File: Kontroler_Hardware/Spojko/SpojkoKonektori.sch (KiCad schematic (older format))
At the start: 14 parts, among them J3 CONN_02X40, J4 CONN_02X40, J5 CONN_02X40, J6 CONN_02X40, J7 CONN_02X40, J8 CONN_02X40

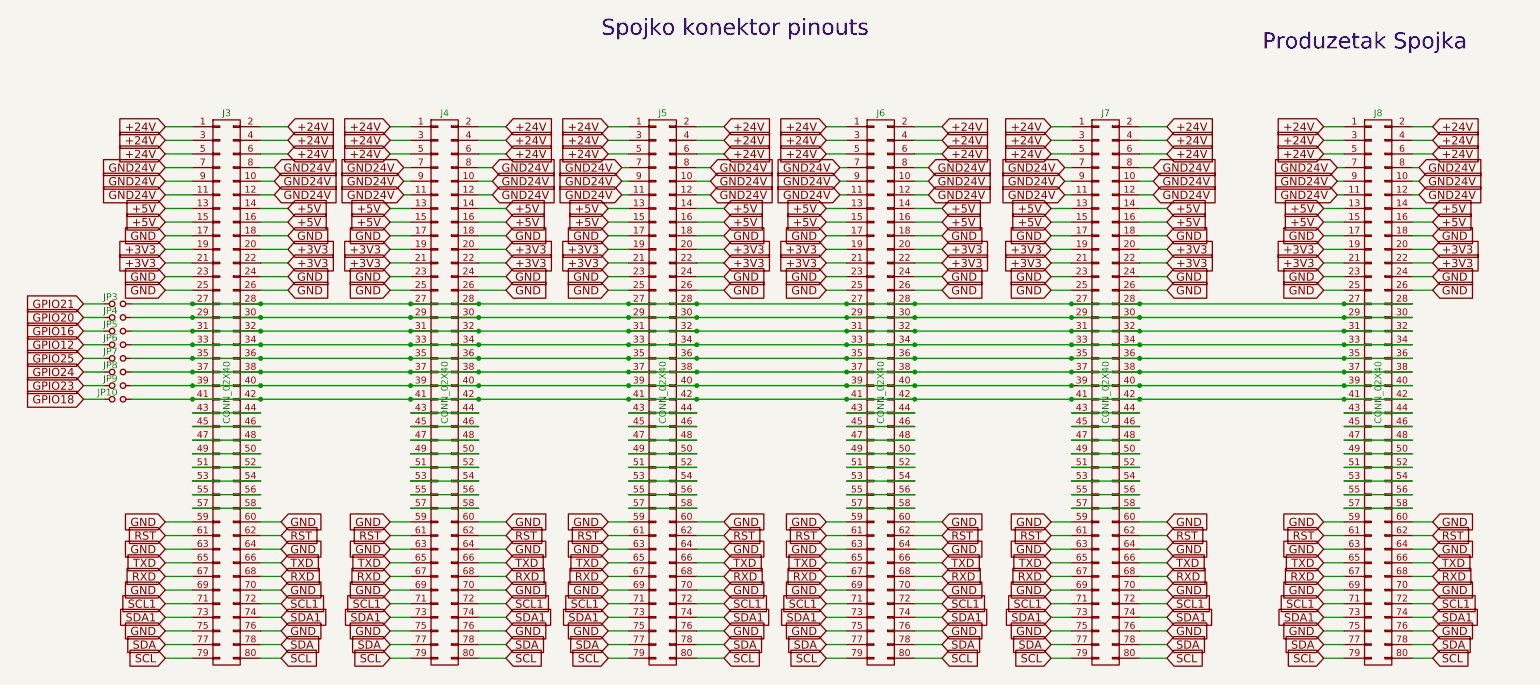
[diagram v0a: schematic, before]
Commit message: NewTemplates
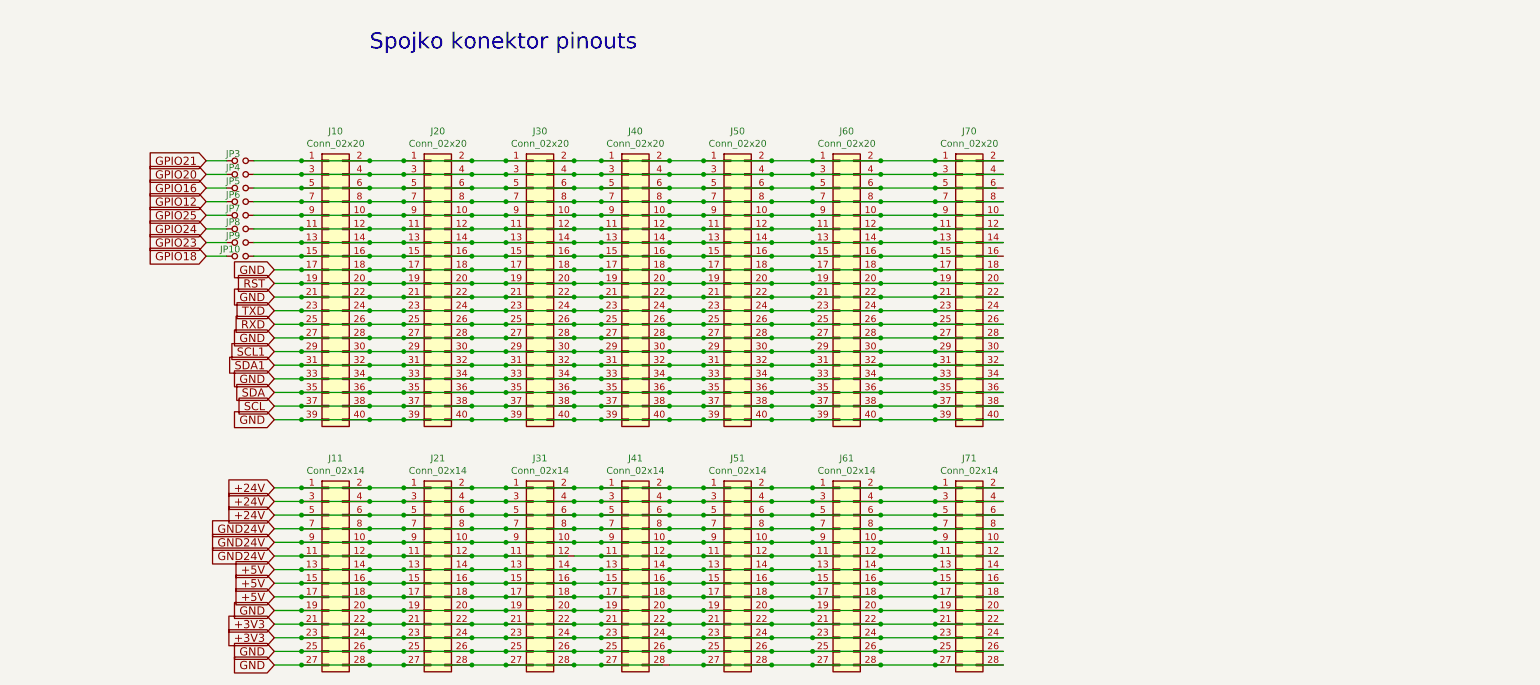
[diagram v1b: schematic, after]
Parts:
- removed J3, J4, J5, J6, J7: CONN_02X40, Pin_Headers:Pin_Header_Straight_2x40_Pitch2.54mm, symbol Spojko-rescue:CONN_02X40
- removed J8: CONN_02X40, Pin_Headers:Pin_Header_Angled_2x40_Pitch2.54mm, symbol Spojko-rescue:CONN_02X40
- added J10, J20, J30, J40, J50, J60: Conn_02x20, Connector_PinHeader_2.54mm:PinHeader_2x20_P2.54mm_Vertical, symbol Spojko-rescue:Conn_02x20_Odd_Even-Connector_Generic
- added J11, J21, J31, J41, J51, J61: Conn_02x14, Connector_PinHeader_2.54mm:PinHeader_2x14_P2.54mm_Vertical, symbol Spojko-rescue:Conn_02x14_Odd_Even-Connector_Generic
- added J70: Conn_02x20, Connector_PinHeader_2.54mm:PinHeader_2x20_P2.54mm_Horizontal, symbol Spojko-rescue:Conn_02x20_Odd_Even-Connector_Generic
- added J71: Conn_02x14, Connector_PinHeader_2.54mm:PinHeader_2x14_P2.54mm_Horizontal, symbol Spojko-rescue:Conn_02x14_Odd_Even-Connector_Generic
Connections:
- net +24V: now also J11.1 (Pin_1), J11.2 (Pin_2), J11.3 (Pin_3), J11.4 (Pin_4), J11.5 (Pin_5), J11.6 (Pin_6), J21.1 (Pin_1), J21.2 (Pin_2), J21.3 (Pin_3), J21.4 (Pin_4), J21.5 (Pin_5), J21.6 (Pin_6), J31.1 (Pin_1), J31.2 (Pin_2), J31.3 (Pin_3), J31.4 (Pin_4), J31.5 (Pin_5), J31.6 (Pin_6), J41.1 (Pin_1), J41.2 (Pin_2), J41.3 (Pin_3), J41.4 (Pin_4), J41.5 (Pin_5), J41.6 (Pin_6), J51.1 (Pin_1), J51.2 (Pin_2), J51.3 (Pin_3), J51.4 (Pin_4), J51.5 (Pin_5), J51.6 (Pin_6), J61.1 (Pin_1), J61.2 (Pin_2), J61.3 (Pin_3), J61.4 (Pin_4), J61.5 (Pin_5), J61.6 (Pin_6), J71.1 (Pin_1), J71.2 (Pin_2), J71.3 (Pin_3), J71.4 (Pin_4), J71.5 (Pin_5), J71.6 (Pin_6)
- net +3V3: now also J11.21 (Pin_21), J11.22 (Pin_22), J11.23 (Pin_23), J11.24 (Pin_24), J21.21 (Pin_21), J21.22 (Pin_22), J21.23 (Pin_23), J21.24 (Pin_24), J31.21 (Pin_21), J31.22 (Pin_22), J31.23 (Pin_23), J31.24 (Pin_24), J41.21 (Pin_21), J41.22 (Pin_22), J41.23 (Pin_23), J41.24 (Pin_24), J51.21 (Pin_21), J51.22 (Pin_22), J51.23 (Pin_23), J51.24 (Pin_24), J61.21 (Pin_21), J61.22 (Pin_22), J61.23 (Pin_23), J61.24 (Pin_24), J71.21 (Pin_21), J71.22 (Pin_22), J71.23 (Pin_23), J71.24 (Pin_24)
- net +5V: now also J11.13 (Pin_13), J11.14 (Pin_14), J11.15 (Pin_15), J11.16 (Pin_16), J11.17 (Pin_17), J11.18 (Pin_18), J21.13 (Pin_13), J21.14 (Pin_14), J21.15 (Pin_15), J21.16 (Pin_16), J21.17 (Pin_17), J21.18 (Pin_18), J31.13 (Pin_13), J31.14 (Pin_14), J31.15 (Pin_15), J31.16 (Pin_16), J31.17 (Pin_17), J31.18 (Pin_18), J41.13 (Pin_13), J41.14 (Pin_14), J41.15 (Pin_15), J41.16 (Pin_16), J41.17 (Pin_17), J41.18 (Pin_18), J51.13 (Pin_13), J51.14 (Pin_14), J51.15 (Pin_15), J51.16 (Pin_16), J51.17 (Pin_17), J51.18 (Pin_18), J61.13 (Pin_13), J61.14 (Pin_14), J61.15 (Pin_15), J61.16 (Pin_16), J61.17 (Pin_17), J61.18 (Pin_18), J71.13 (Pin_13), J71.14 (Pin_14), J71.15 (Pin_15), J71.16 (Pin_16), J71.17 (Pin_17), J71.18 (Pin_18)
- net GND: now also J10.17 (Pin_17), J10.18 (Pin_18), J10.21 (Pin_21), J10.22 (Pin_22), J10.27 (Pin_27), J10.28 (Pin_28), J10.33 (Pin_33), J10.34 (Pin_34), J10.39 (Pin_39), J10.40 (Pin_40), J11.19 (Pin_19), J11.20 (Pin_20), J11.25 (Pin_25), J11.26 (Pin_26), J11.27 (Pin_27), J11.28 (Pin_28), J20.17 (Pin_17), J20.18 (Pin_18), J20.21 (Pin_21), J20.22 (Pin_22), J20.27 (Pin_27), J20.28 (Pin_28), J20.33 (Pin_33), J20.34 (Pin_34), J20.39 (Pin_39), J20.40 (Pin_40), J21.19 (Pin_19), J21.20 (Pin_20), J21.25 (Pin_25), J21.26 (Pin_26), J21.27 (Pin_27), J21.28 (Pin_28), J30.17 (Pin_17), J30.18 (Pin_18), J30.21 (Pin_21), J30.22 (Pin_22), J30.27 (Pin_27), J30.28 (Pin_28), J30.33 (Pin_33), J30.34 (Pin_34), J30.39 (Pin_39), J30.40 (Pin_40), J31.19 (Pin_19), J31.20 (Pin_20), J31.25 (Pin_25), J31.26 (Pin_26), J31.27 (Pin_27), J31.28 (Pin_28), J40.17 (Pin_17), J40.18 (Pin_18), J40.21 (Pin_21), J40.22 (Pin_22), J40.27 (Pin_27), J40.28 (Pin_28), J40.33 (Pin_33), J40.34 (Pin_34), J40.39 (Pin_39), J40.40 (Pin_40), J41.19 (Pin_19), J41.20 (Pin_20), J41.25 (Pin_25), J41.26 (Pin_26), J41.27 (Pin_27), J50.17 (Pin_17), J50.18 (Pin_18), J50.21 (Pin_21), J50.22 (Pin_22), J50.27 (Pin_27), J50.28 (Pin_28), J50.33 (Pin_33), J50.34 (Pin_34), J50.39 (Pin_39), J50.40 (Pin_40), J51.19 (Pin_19), J51.20 (Pin_20), J51.25 (Pin_25), J51.26 (Pin_26), J60.17 (Pin_17), J60.18 (Pin_18), J60.21 (Pin_21), J60.22 (Pin_22), J60.27 (Pin_27), J60.28 (Pin_28), J60.33 (Pin_33), J60.34 (Pin_34), J60.39 (Pin_39), J60.40 (Pin_40), J61.19 (Pin_19), J61.20 (Pin_20), J61.25 (Pin_25), J61.26 (Pin_26), J70.17 (Pin_17), J70.18 (Pin_18), J70.21 (Pin_21), J70.22 (Pin_22), J70.27 (Pin_27), J70.28 (Pin_28), J70.33 (Pin_33), J70.34 (Pin_34), J70.39 (Pin_39), J70.40 (Pin_40), J71.19 (Pin_19), J71.20 (Pin_20), J71.25 (Pin_25), J71.26 (Pin_26)
- net GND24V: now also J11.10 (Pin_10), J11.11 (Pin_11), J11.12 (Pin_12), J11.7 (Pin_7), J11.8 (Pin_8), J11.9 (Pin_9), J21.10 (Pin_10), J21.11 (Pin_11), J21.12 (Pin_12), J21.7 (Pin_7), J21.8 (Pin_8), J21.9 (Pin_9), J31.10 (Pin_10), J31.11 (Pin_11), J31.7 (Pin_7), J31.8 (Pin_8), J31.9 (Pin_9), J41.10 (Pin_10), J41.7 (Pin_7), J41.8 (Pin_8), J41.9 (Pin_9), J51.10 (Pin_10), J51.7 (Pin_7), J51.8 (Pin_8), J51.9 (Pin_9), J61.10 (Pin_10), J61.7 (Pin_7), J61.8 (Pin_8), J61.9 (Pin_9), J71.10 (Pin_10), J71.7 (Pin_7), J71.8 (Pin_8), J71.9 (Pin_9)
- net RST: now also J10.19 (Pin_19), J10.20 (Pin_20), J20.19 (Pin_19), J20.20 (Pin_20), J30.19 (Pin_19), J30.20 (Pin_20), J40.19 (Pin_19), J40.20 (Pin_20), J50.19 (Pin_19), J50.20 (Pin_20), J60.19 (Pin_19), J60.20 (Pin_20), J70.19 (Pin_19), J70.20 (Pin_20)
- net RXD: now also J10.25 (Pin_25), J10.26 (Pin_26), J20.25 (Pin_25), J20.26 (Pin_26), J30.25 (Pin_25), J30.26 (Pin_26), J40.25 (Pin_25), J40.26 (Pin_26), J50.25 (Pin_25), J50.26 (Pin_26), J60.25 (Pin_25), J60.26 (Pin_26), J70.25 (Pin_25), J70.26 (Pin_26)
- net SCL: now also J10.37 (Pin_37), J10.38 (Pin_38), J20.37 (Pin_37), J20.38 (Pin_38), J30.37 (Pin_37), J30.38 (Pin_38), J40.37 (Pin_37), J40.38 (Pin_38), J50.37 (Pin_37), J50.38 (Pin_38), J60.37 (Pin_37), J60.38 (Pin_38), J70.37 (Pin_37), J70.38 (Pin_38)
- net SCL1: now also J10.29 (Pin_29), J10.30 (Pin_30), J20.29 (Pin_29), J20.30 (Pin_30), J30.29 (Pin_29), J30.30 (Pin_30), J40.29 (Pin_29), J40.30 (Pin_30), J50.29 (Pin_29), J50.30 (Pin_30), J60.29 (Pin_29), J60.30 (Pin_30), J70.29 (Pin_29), J70.30 (Pin_30)
- net SDA: now also J10.35 (Pin_35), J10.36 (Pin_36), J20.35 (Pin_35), J20.36 (Pin_36), J30.35 (Pin_35), J30.36 (Pin_36), J40.35 (Pin_35), J40.36 (Pin_36), J50.35 (Pin_35), J50.36 (Pin_36), J60.35 (Pin_35), J60.36 (Pin_36), J70.35 (Pin_35), J70.36 (Pin_36)
- net SDA1: now also J10.31 (Pin_31), J10.32 (Pin_32), J20.31 (Pin_31), J20.32 (Pin_32), J30.31 (Pin_31), J30.32 (Pin_32), J40.31 (Pin_31), J40.32 (Pin_32), J50.31 (Pin_31), J50.32 (Pin_32), J60.31 (Pin_31), J60.32 (Pin_32), J70.31 (Pin_31), J70.32 (Pin_32)
- net TXD: now also J10.23 (Pin_23), J10.24 (Pin_24), J20.23 (Pin_23), J20.24 (Pin_24), J30.23 (Pin_23), J30.24 (Pin_24), J40.23 (Pin_23), J40.24 (Pin_24), J50.23 (Pin_23), J50.24 (Pin_24), J60.23 (Pin_23), J60.24 (Pin_24), J70.23 (Pin_23), J70.24 (Pin_24)
- net at JP3.2: now also J10.1 (Pin_1), J10.2 (Pin_2), J20.1 (Pin_1), J20.2 (Pin_2), J30.1 (Pin_1), J30.2 (Pin_2), J40.1 (Pin_1), J40.2 (Pin_2), J50.1 (Pin_1), J50.2 (Pin_2), J60.1 (Pin_1), J60.2 (Pin_2), J70.1 (Pin_1), J70.2 (Pin_2)
- net at JP4.2: now also J10.3 (Pin_3), J10.4 (Pin_4), J20.3 (Pin_3), J20.4 (Pin_4), J30.3 (Pin_3), J30.4 (Pin_4), J40.3 (Pin_3), J40.4 (Pin_4), J50.3 (Pin_3), J50.4 (Pin_4), J60.3 (Pin_3), J60.4 (Pin_4), J70.3 (Pin_3), J70.4 (Pin_4)
- net at JP5.2: now also J10.5 (Pin_5), J10.6 (Pin_6), J20.5 (Pin_5), J20.6 (Pin_6), J30.5 (Pin_5), J30.6 (Pin_6), J40.5 (Pin_5), J40.6 (Pin_6), J50.5 (Pin_5), J50.6 (Pin_6), J60.5 (Pin_5), J60.6 (Pin_6), J70.5 (Pin_5)
- net at JP6.2: now also J10.7 (Pin_7), J10.8 (Pin_8), J20.7 (Pin_7), J20.8 (Pin_8), J30.7 (Pin_7), J30.8 (Pin_8), J40.7 (Pin_7), J40.8 (Pin_8), J50.7 (Pin_7), J50.8 (Pin_8), J60.7 (Pin_7), J60.8 (Pin_8), J70.7 (Pin_7), J70.8 (Pin_8)
- net at JP7.2: now also J10.10 (Pin_10), J10.9 (Pin_9), J20.10 (Pin_10), J20.9 (Pin_9), J30.10 (Pin_10), J30.9 (Pin_9), J40.10 (Pin_10), J40.9 (Pin_9), J50.10 (Pin_10), J50.9 (Pin_9), J60.10 (Pin_10), J60.9 (Pin_9), J70.10 (Pin_10), J70.9 (Pin_9)
- net at JP8.2: now also J10.11 (Pin_11), J10.12 (Pin_12), J20.11 (Pin_11), J20.12 (Pin_12), J30.11 (Pin_11), J30.12 (Pin_12), J40.11 (Pin_11), J40.12 (Pin_12), J50.11 (Pin_11), J50.12 (Pin_12), J60.11 (Pin_11), J60.12 (Pin_12), J70.11 (Pin_11), J70.12 (Pin_12)
- net at JP9.2: now also J10.13 (Pin_13), J10.14 (Pin_14), J20.13 (Pin_13), J20.14 (Pin_14), J30.13 (Pin_13), J30.14 (Pin_14), J40.13 (Pin_13), J40.14 (Pin_14), J50.13 (Pin_13), J50.14 (Pin_14), J60.13 (Pin_13), J60.14 (Pin_14), J70.13 (Pin_13), J70.14 (Pin_14)
- net at JP10.2: now also J10.15 (Pin_15), J10.16 (Pin_16), J20.15 (Pin_15), J20.16 (Pin_16), J30.15 (Pin_15), J30.16 (Pin_16), J40.15 (Pin_15), J40.16 (Pin_16), J50.15 (Pin_15), J50.16 (Pin_16), J60.15 (Pin_15), J60.16 (Pin_16), J70.15 (Pin_15)
- new net: J31.12 (Pin_12), J41.11 (Pin_11), J41.12 (Pin_12), J51.11 (Pin_11), J51.12 (Pin_12), J61.11 (Pin_11), J61.12 (Pin_12), J71.11 (Pin_11), J71.12 (Pin_12)
- new net: J41.28 (Pin_28), J51.27 (Pin_27), J51.28 (Pin_28), J61.27 (Pin_27), J61.28 (Pin_28), J71.27 (Pin_27), J71.28 (Pin_28)
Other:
- note removed: "Produzetak Spojka\n"
- moved on the sheet: JP10, JP3, JP4, JP5, JP6, JP7, JP8, JP9
